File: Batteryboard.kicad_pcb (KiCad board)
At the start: 4 copper layers, 76.2 x 76.2 mm, 148 parts, among them IC1 FAN4010IL6X_F113, IC2 FAN4010IL6X_F113, IC3 FAN4010IL6X_F113, J1 Conn_01x02_Male, J2 Conn_01x03_Male, J3 Conn_01x05_Male, J4 Conn_01x02_Male, J5 SC_19-20, Q1 SI7617DN-T1-GE3, Q2 SI7617DN-T1-GE3, Q3 SI7617DN-T1-GE3, Q4 SIS412DN-T1-GE3, Q5 SIS412DN-T1-GE3, Q6 SIS412DN-T1-GE3, Q7 SI7617DN-T1-GE3, Q8 SIS412DN-T1-GE3, U1 BQ24617RGET, U2 TPS65279DAPR, U3 BQ29200DRBT, U4 PIC18F25K50-I_SO, U5 MCP2515-xSO, U6 SN65HVD1050D

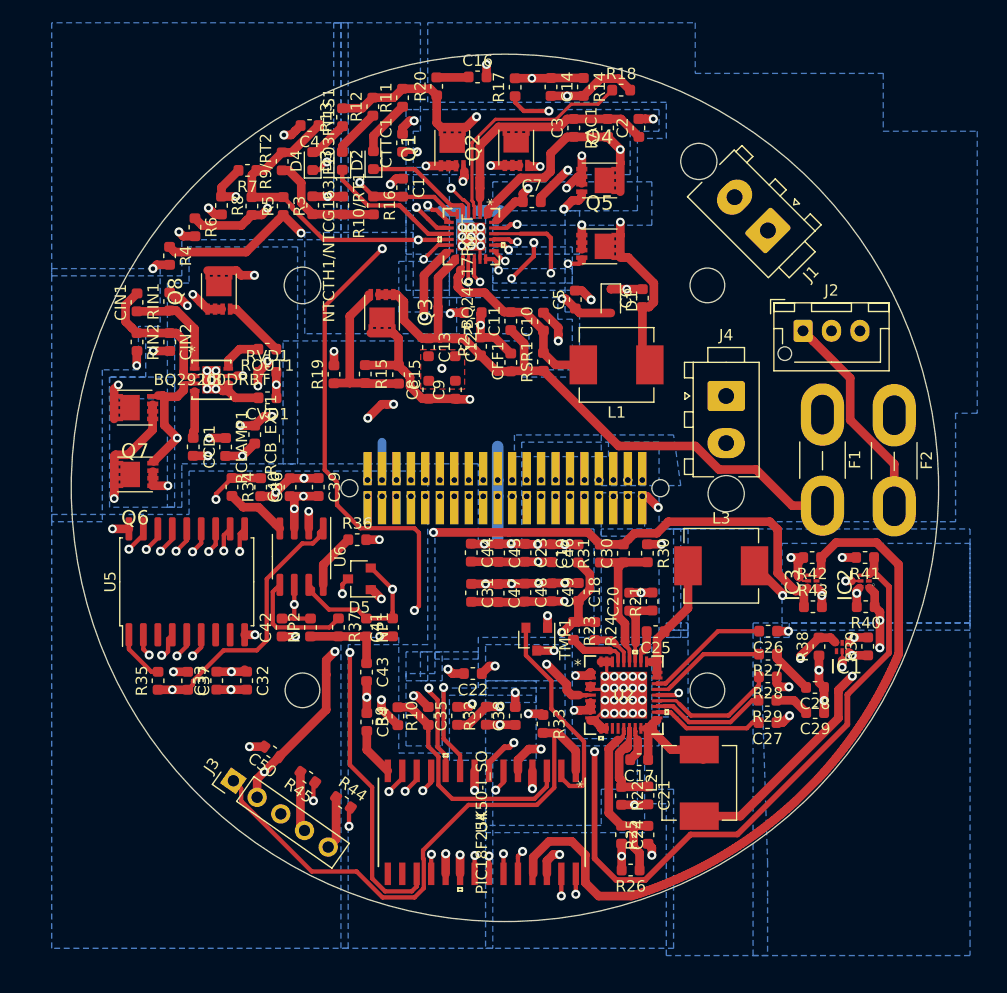
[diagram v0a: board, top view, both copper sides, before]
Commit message: big overhaul on board, did a bunch of stuff
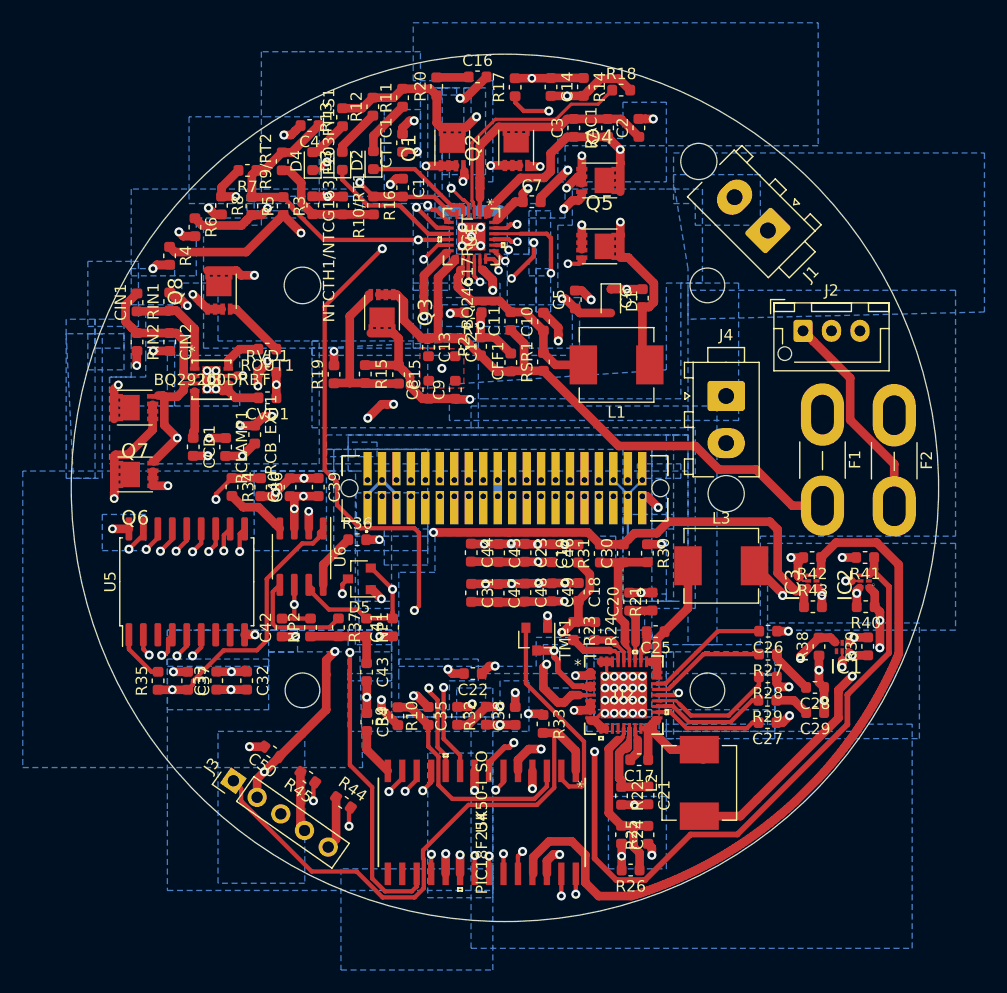
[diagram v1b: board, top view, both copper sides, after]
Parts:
- C20, C21, C34, C35, C38, C50: value C -> .1uF
- C26, C27: value C -> 50nF
- J5: footprint MASA-LIB:bottom_Stack_Connector_2019_2020 -> MASA-LIB:Stack_Connector_2019_2020
- R10, R32, R9: value R_US -> 10kOhm
- R21, R22: value R_US -> 60.4kOhm
- R28: value R_US -> 30Ohm
- R33: value R_US -> 470Ohm
- R44, R45: value R_US -> 100Ohm
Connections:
- C1 pad 1: PGND2 -> VSS
- C10 pad 2: PGND2 -> VSS
- C2 pad 2: PGND2 -> VSS
- C20 pad 2: PGND2 -> VSS
- C21 pad 2: PGND2 -> VSS
- C26 pad 1: PGND2 -> VSS
- C27 pad 1: PGND2 -> VSS
- C28 pad 1: PGND2 -> VSS
- C29 pad 1: PGND2 -> VSS
- C32 pad 2: PGND2 -> VSS
- C33 pad 1: PGND2 -> VSS
- C34 pad 1: PGND2 -> VSS
- C35 pad 2: PGND2 -> VSS
- C36 pad 2: PGND2 -> VSS
- C37 pad 1: PGND2 -> VSS
- C38 pad 2: PGND2 -> VSS
- C39 pad 1: PGND2 -> VSS
- C4 pad 2: PGND2 -> VSS
- C40 pad 2: PGND2 -> VSS
- C41 pad 1: PGND2 -> VSS
- C42 pad 1: PGND2 -> VSS
- C43 pad 2: PGND2 -> VSS
- C50 pad 2: PGND2 -> VSS
- C7 pad 2: PGND2 -> VSS
- CTTC1 pad 2: PGND2 -> VSS
- D5 pad 1: PGND2 -> VSS
- IC1 pad 5: PGND2 -> VSS
- IC2 pad 5: PGND2 -> VSS
- IC3 pad 5: PGND2 -> VSS
- J3 pad 3: PGND2 -> VSS
- J5 pad 1: PGND2 -> VSS
- J5 pad 19: PGND2 -> VSS
- J5 pad 20: PGND2 -> VSS
- J5 pad 36: PGND2 -> VSS
- J5 pad 37: PGND2 -> VSS
- J5 pad 4: PGND2 -> VSS
- J5 pad 40: PGND2 -> VSS
- J5 pad 5: PGND2 -> VSS
- NTCTH1/NTCG163JF103FT1S1 pad 1: PGND2 -> VSS
- R1 pad 2: PGND2 -> VSS
- R10/RT1 pad 1: PGND2 -> VSS
- R21 pad 2: PGND2 -> VSS
- R22 pad 2: PGND2 -> VSS
- R25 pad 1: PGND2 -> VSS
- R28 pad 1: PGND2 -> VSS
- R30 pad 1: PGND2 -> VSS
- R36 pad 2: PGND2 -> VSS
- R38 pad 1: PGND2 -> VSS
- R4 pad 2: PGND2 -> VSS
- R41 pad 2: PGND2 -> VSS
- R42 pad 2: PGND2 -> VSS
- R6 pad 2: PGND2 -> VSS
- R8 pad 2: PGND2 -> VSS
- R_JUMP1 pad 1: PGND2 -> VSS
- TMP1 pad 3: PGND2 -> VSS
- U1 pad 25: PGND2 -> VSS
- U2 pad 23: PGND2 -> VSS
- U2 pad 3: PGND2 -> VSS
- U2 pad 4: PGND2 -> VSS
- U4 pad 19: PGND2 -> VSS
- U4 pad 8: PGND2 -> VSS
- U5 pad 18: PGND2 -> VSS
- U6 pad 2: PGND2 -> VSS
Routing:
- net VSS: track 0.00 -> 113.3 mm, vias 0 -> 47
- net PGND2: track 156.1 -> 57.7 mm, vias 94 -> 44
- net V7V: track 12.4 -> 14.3 mm
- net Net-(R19-Pad2): track 27.8 -> 28.9 mm
- net CAN_L: vias 3 -> 2
- net CAN_H: vias 2 -> 1
- net 5V0: vias 15 -> 11
- net 3V3: vias 8 -> 4
- added copper zone on B.Cu, net (none)
- added copper zone on B.Cu, net VSS
